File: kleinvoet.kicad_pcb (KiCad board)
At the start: 4 copper layers, 122 x 66 mm, 189 parts, among them J1 Conn_ST_STDC14, J11 Micro_SD_Card_Det, J12 JST-PH, J13 USB_C_Receptacle_USB2.0, J16 GPS_Transmission_Conn, J2 FTDI_Conn, J3 Sensor_Conn, J4 GPS_Transmission_Conn, J6 Sensor_Conn, Q1 PMOS, SW1 RESET, SW2 USER, U1 STM32F446RETx, U10 USBLC6-2SC6, U11 ublox_SAM-M8Q, U2 ADAU1978, U3 THS4551, U5 THS4551, U8 MCP73831-2-OT, U9 TPS73733QDRBRQ1, X1 12.288MHz, Y1 12 MHz, Y2 32.768 kHz

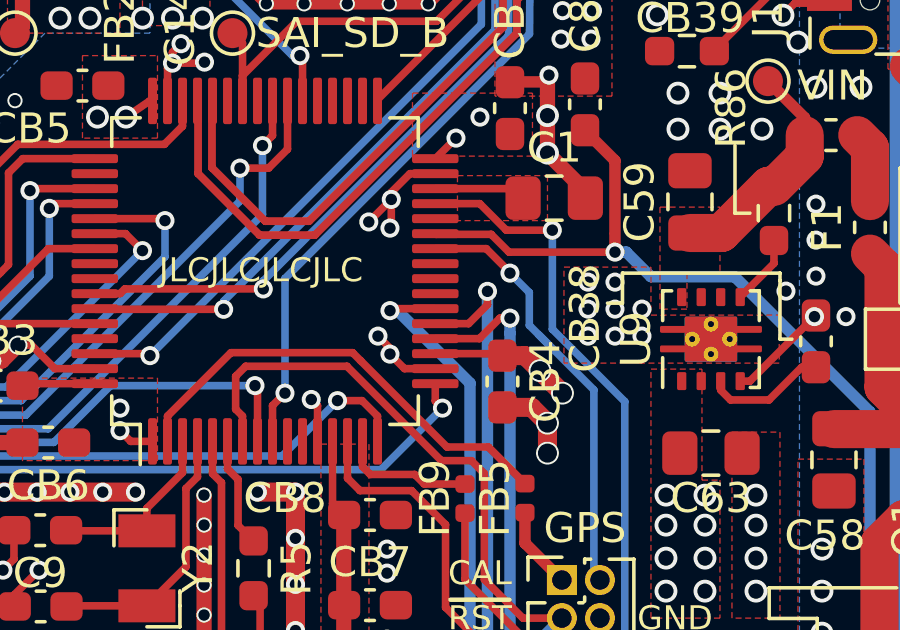
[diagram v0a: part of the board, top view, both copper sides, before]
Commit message: Update pinout
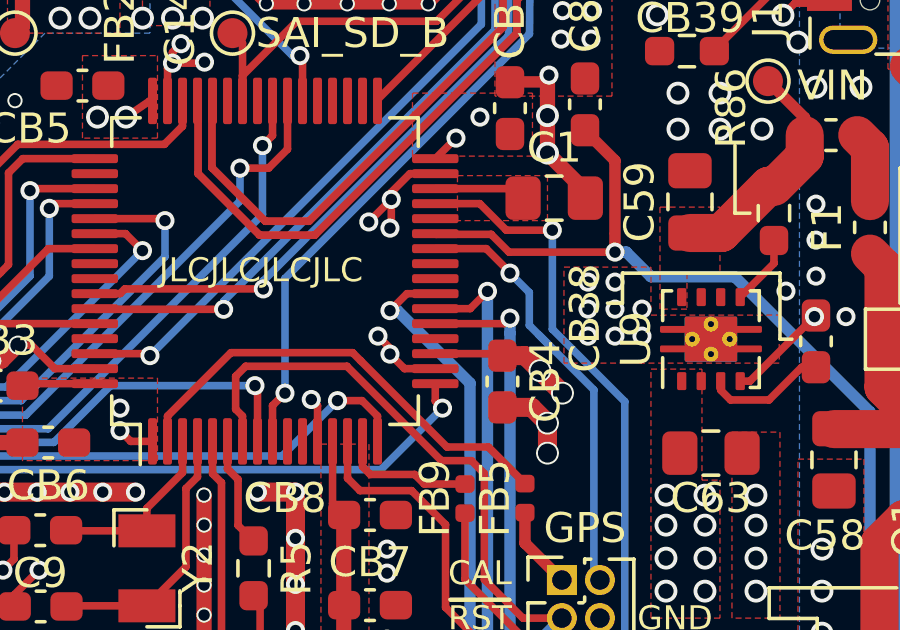
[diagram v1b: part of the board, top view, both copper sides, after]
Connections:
- CB9 pad 1: /D12 -> /D11
- R2 pad 2: /A2 -> /D13
- R8 pad 2: /D13 -> /D12
- SW2 pad 1: /D12 -> /D11
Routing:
- net /D11: track 0.00 -> 73.2 mm, vias 0 -> 2
- net /D12: track 72.9 -> 18.9 mm
- net /A2: track 19.7 -> 0.00 mm, vias 2 -> 0
